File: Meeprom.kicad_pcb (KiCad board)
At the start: 2 copper layers, 16 x 38 mm, 4 parts, among them J1 Molex 8878 socket 27C256 pino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, U1 28C256

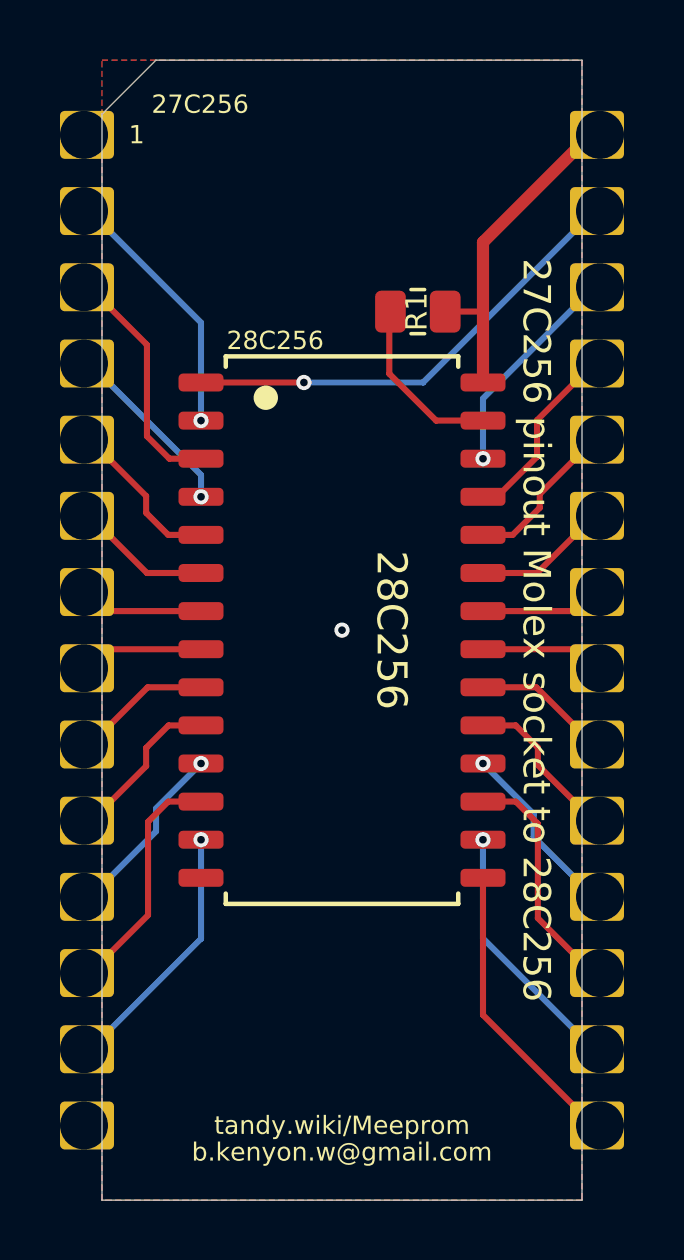
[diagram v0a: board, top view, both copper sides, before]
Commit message: cosmetics
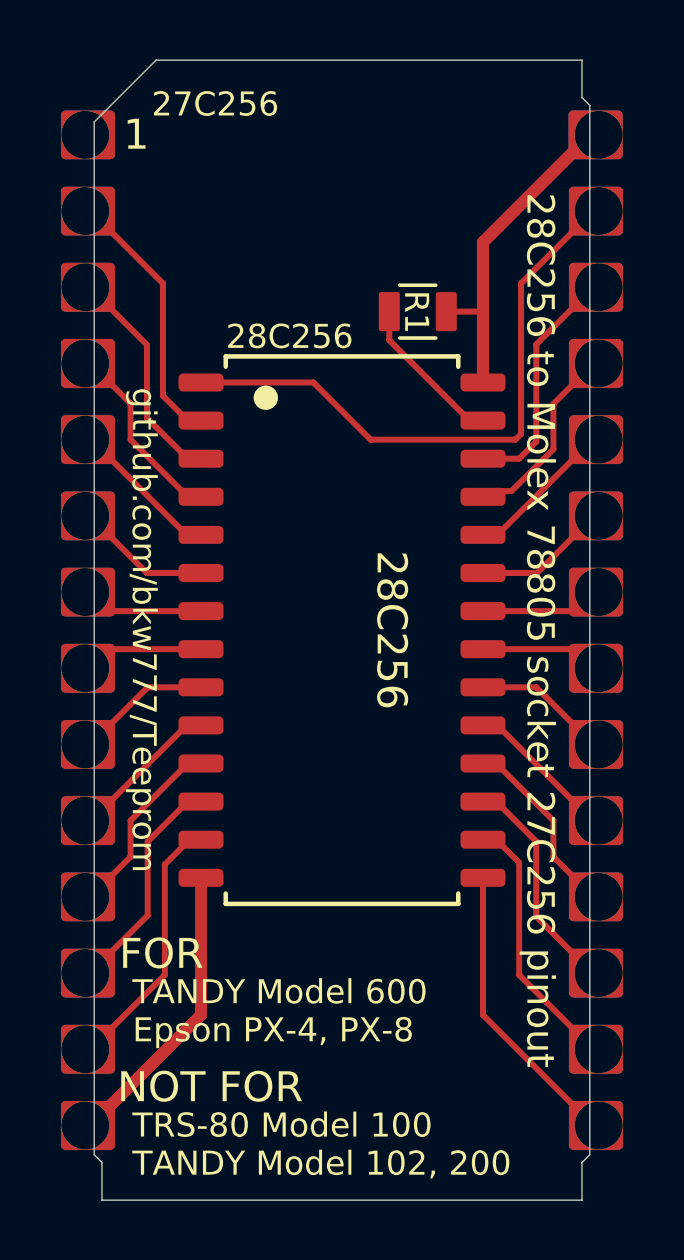
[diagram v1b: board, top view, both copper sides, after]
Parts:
- removed carrier?: pcb2molex8878_chamfer, 000_LOCAL:pcb2molex8878_chamfer
- J1: value Molex 8878 socket 27C256 pinout -> Molex 78805 socket 27C256 pinout; footprint 000_LOCAL:pcb2molex8878 -> 000_LOCAL:Molex78805_PCB
- R1: footprint 000_LOCAL:R_0805_2012Metric -> 000_LOCAL:R_0805
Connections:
- net /VCC renamed VCC
- J1 pad 14: /VSS -> (no net)
- U1 pad 14: /VSS -> (no net)
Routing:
- net (no net): track 0.00 -> 9.95 mm
- net /A14: track 15.7 -> 20.1 mm, vias 1 -> 0
- net /A13: track 7.44 -> 8.12 mm, vias 1 -> 0
- net /~WE: track 5.84 -> 5.19 mm
- net /A6: track 6.08 -> 6.40 mm, vias 1 -> 0
- net /D4: track 8.63 -> 8.94 mm, vias 1 -> 0
- net /D6: track 6.09 -> 6.40 mm, vias 1 -> 0
- net /D0: track 6.10 -> 6.40 mm, vias 1 -> 0
- net /D2: track 8.64 -> 8.91 mm, vias 1 -> 0
- net /A12: track 8.71 -> 8.94 mm, vias 1 -> 0
- net /VSS: vias 1 -> 0
- removed copper zone on B.Cu, net /VSS
- removed copper zone on F.Cu, net /VSS
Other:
- board size 16 x 38 mm -> 16.5 x 38 mm
- net class Default: clearance 0.2032 -> 0.2; trace_width 0.2032 -> 0.2; via_dia 0.508 -> 0.5; via_drill 0.254 -> 0.3
- rule trace_clearance: 0.2032 -> 0.2
- rule trace_min: 0.1524 -> 0.2
- rule via_min_drill: 0.254 -> 0.3
- rule via_min_size: 0.508 -> 0.5
- board text added: "28C256 to Molex 78805 socket 27C256 pinout"
- board text added: "Epson PX-4, PX-8"
- board text added: "FOR"
- board text added: "NOT FOR"
- board text added: "TANDY Model 102, 200"
- board text added: "TANDY Model 600"
- board text added: "TRS-80 Model 100"
- board text added: "Use with carrier: http://shpws.me/RqW3"
- board text added: "github.com/bkw777/Teeprom"
- board text removed: "27C256 pinout Molex socket to 28C256"
- board text removed: "Use with thingiverse.com/thing:3821586"
- board text removed: "b.kenyon.w@gmail.com"
- board text removed: "tandy.wiki/Meeprom"
